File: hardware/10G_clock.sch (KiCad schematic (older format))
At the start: 12 parts, among them U801 DIFF_OSC, U802 DIFF_OSC, U803 SI53340

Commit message: Fixed Schematic Symbols
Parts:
- C801, C802, C805: symbol device:C -> Device:C_Small
- C803, C804: symbol device:C_Small -> Device:C_Small
- R801, R802, R803, R804: symbol device:R -> Device:R
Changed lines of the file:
@@
 $Descr A4 11693 8268
 encoding utf-8
-Sheet 8 22
+Sheet 8 21
 Title ""
 Date ""
@@
 Note: clocks are AC-coupled at receiving device.
 $Comp
-L power1:GND #PWR084
+L power:GND #PWR084
 U 1 1 598A8A47
 P 1700 2300
@@
 NoConn ~ 5500 4800
 $Comp
-L device:C_Small C803
+L Device:C_Small C803
 U 1 1 598F26F6
 P 3500 3900
@@
 $EndComp
 $Comp
-L device:C_Small C804
+L Device:C_Small C804
 U 1 1 598F2737
 P 3500 4200
@@
 $EndComp
 $Comp
-L device:R R804
+L Device:R R804
 U 1 1 598F277A
 P 3700 4050
@@
 Connection ~ 3700 4200
 $Comp
-L device:C C802
+L Device:C_Small C802
 U 1 1 598F29AD
 P 3350 3250
@@
 $EndComp
 $Comp
-L power1:GND #PWR085
+L power:GND #PWR085
 U 1 1 598F2A12
 P 3350 3400
@@
 $EndComp
 $Comp
-L power1:+3V3 #PWR086
+L power:+3V3 #PWR086
 U 1 1 598F2A6C
 P 3200 3000
@@
 	3300 4200 3400 4200
 $Comp
-L device:C C805
+L Device:C_Small C805
 U 1 1 598F30AD
 P 4900 3300
@@
 $EndComp
 $Comp
-L power1:GND #PWR087
+L power:GND #PWR087
 U 1 1 598F3107
 P 4900 3450
@@
 $EndComp
 $Comp
-L power1:+3V3 #PWR088
+L power:+3V3 #PWR088
 U 1 1 598F312D
 P 4700 3050
@@
 Connection ~ 4700 3150
 $Comp
-L device:C C801
+L Device:C_Small C801
 U 1 1 598F396E
 P 3350 1550
@@
 $EndComp
 $Comp
-L power1:GND #PWR089
+L power:GND #PWR089
 U 1 1 598F3974
 P 3350 1700
@@
 $EndComp
 $Comp
-L power1:+3V3 #PWR090
+L power:+3V3 #PWR090
 U 1 1 598F397A
 P 3200 1300
@@
 Connection ~ 3200 1400
 $Comp
-L power1:GND #PWR091
+L power:GND #PWR091
 U 1 1 598F433B
 P 1700 4000
@@
 NoConn ~ 1800 3500
 $Comp
-L power1:GND #PWR092
+L power:GND #PWR092
 U 1 1 598F54B6
 P 4800 5200
@@
 	3900 3900 3900 4100
 $Comp
-L power1:GND #PWR093
+L power:GND #PWR093
 U 1 1 598F5D66
 P 2350 4400
@@
 $EndComp
 $Comp
-L power1:+3V3 #PWR094
+L power:+3V3 #PWR094
 U 1 1 598F5D8C
 P 2150 4500
@@
 $EndComp
 $Comp
-L power1:GND #PWR095
+L power:GND #PWR095
 U 1 1 598F5DE1
 P 2350 4700
@@
 $EndComp
 $Comp
-L device:R R801
+L Device:R R801
 U 1 1 598F6241
 P 2500 4400
@@
 $EndComp
 $Comp
-L device:R R803
+L Device:R R803
 U 1 1 598F6296
 P 2800 4500
@@
 $EndComp
 $Comp
-L device:R R802
+L Device:R R802
 U 1 1 598F62E9
 P 2500 4700

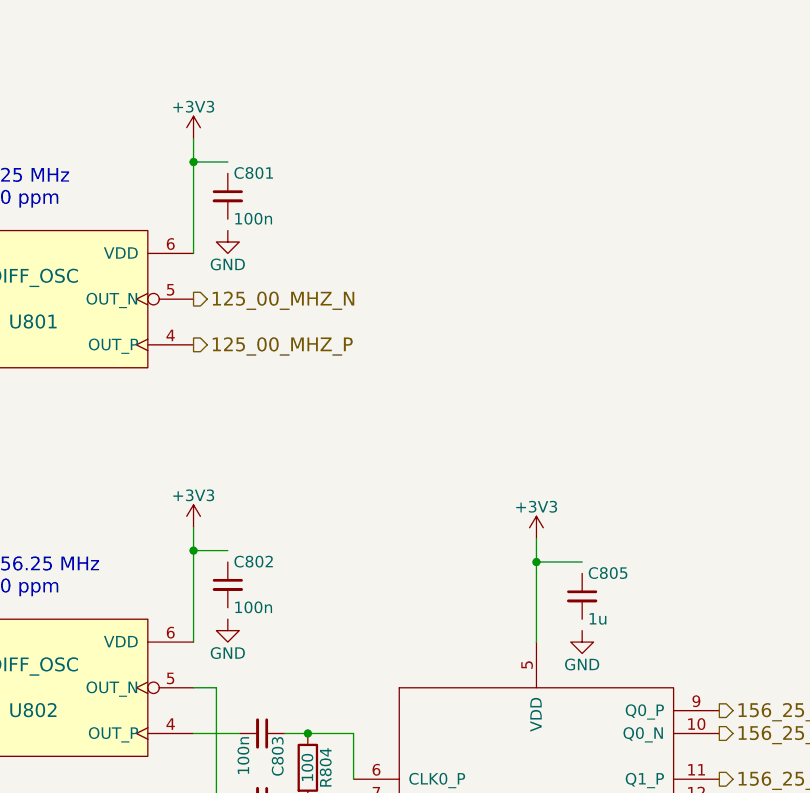
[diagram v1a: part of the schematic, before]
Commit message: WIP: TLK Powerdistribution
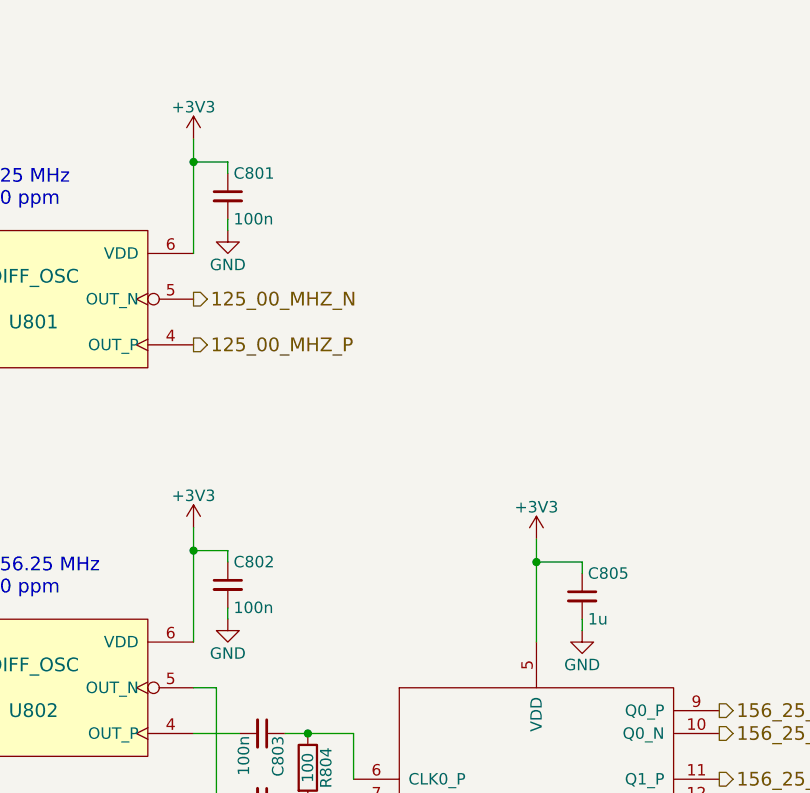
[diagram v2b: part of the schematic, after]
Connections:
- wire segments 31 -> 37
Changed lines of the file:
@@
 EESchema Schematic File Version 4
-LIBS:zynq_board-cache
 EELAYER 26 0
 EELAYER END
 $Descr A4 11693 8268
 encoding utf-8
-Sheet 8 21
+Sheet 7 21
 Title ""
 Date ""
@@
 Wire Wire Line
 	4800 5150 4900 5150
+Wire Wire Line
+	3350 1400 3350 1450
+Wire Wire Line
+	3350 1650 3350 1700
+Wire Wire Line
+	3350 3150 3350 3100
+Wire Wire Line
+	3350 3350 3350 3400
+Wire Wire Line
+	4900 3200 4900 3150
+Wire Wire Line
+	4900 3400 4900 3450
 $EndSCHEMATC
